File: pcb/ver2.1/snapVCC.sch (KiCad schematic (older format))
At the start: 16 parts, among them P1 CONN_01X03, P2 CONN_01X02, Q1 IRLML9301TRPbF, U1 TPS560200

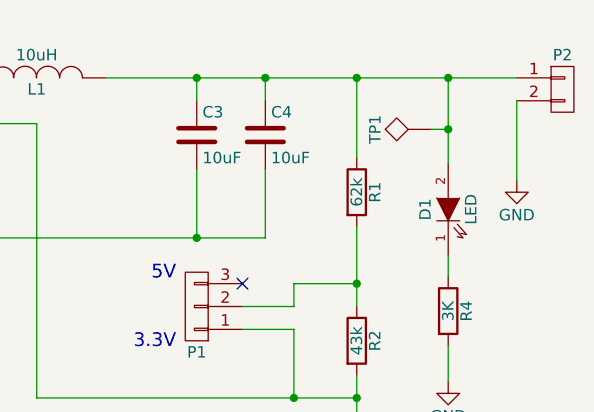
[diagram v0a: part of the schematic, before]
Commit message: changes updated
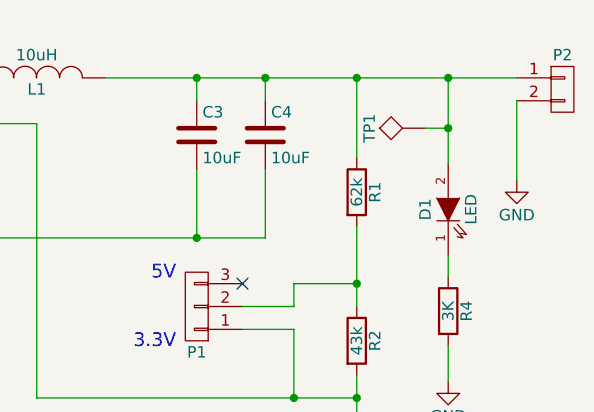
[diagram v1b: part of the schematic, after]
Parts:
- TP1: footprint snapVCC_lib:0R -> (none)
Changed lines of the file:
@@
 $Comp
 L TEST TP1
-U 1 1 598997EE
-P 8280 3140
-F 0 "TP1" H 8280 3355 50  0000 C BNN
-F 1 "TEST" H 8280 3390 50  0001 C CNN
-F 2 "snapVCC_lib:0R" H 8280 3140 50  0001 C CNN
-F 3 "" H 8280 3140 50  0001 C CNN
-	1    8280 3140
+U 1 1 5989908A
+P 8255 3135
+F 0 "TP1" H 8255 3350 50  0000 C BNN
+F 1 "TEST" H 8255 3385 50  0001 C CNN
+F 2 "" H 8255 3135 50  0001 C CNN
+F 3 "" H 8255 3135 50  0001 C CNN
+	1    8255 3135
 	0    -1   -1   0
 $EndComp
 Wire Wire Line
-	8280 3140 8355 3140
-Connection ~ 8355 3140
+	8255 3135 8355 3135
+Connection ~ 8355 3135
 $EndSCHEMATC
